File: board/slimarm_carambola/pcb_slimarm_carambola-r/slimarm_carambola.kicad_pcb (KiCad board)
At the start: 4 copper layers, 50 x 29.7 mm, 85 parts, among them J1 USB_C_Receptacle_USB2.0, J2 Conn_01x14_Pin, J3 Micro_SD_Card_Det2, J4 DF13A-7P-1.25H21, J5 Conn_01x03, U1 AT91SAM9G25-CU, U2 16bit-DDR2-8bank-FBGA84, U3 SY8089AAAC, U5 AMS1117, U7 XC6206PxxxMR, Y1 Crystal

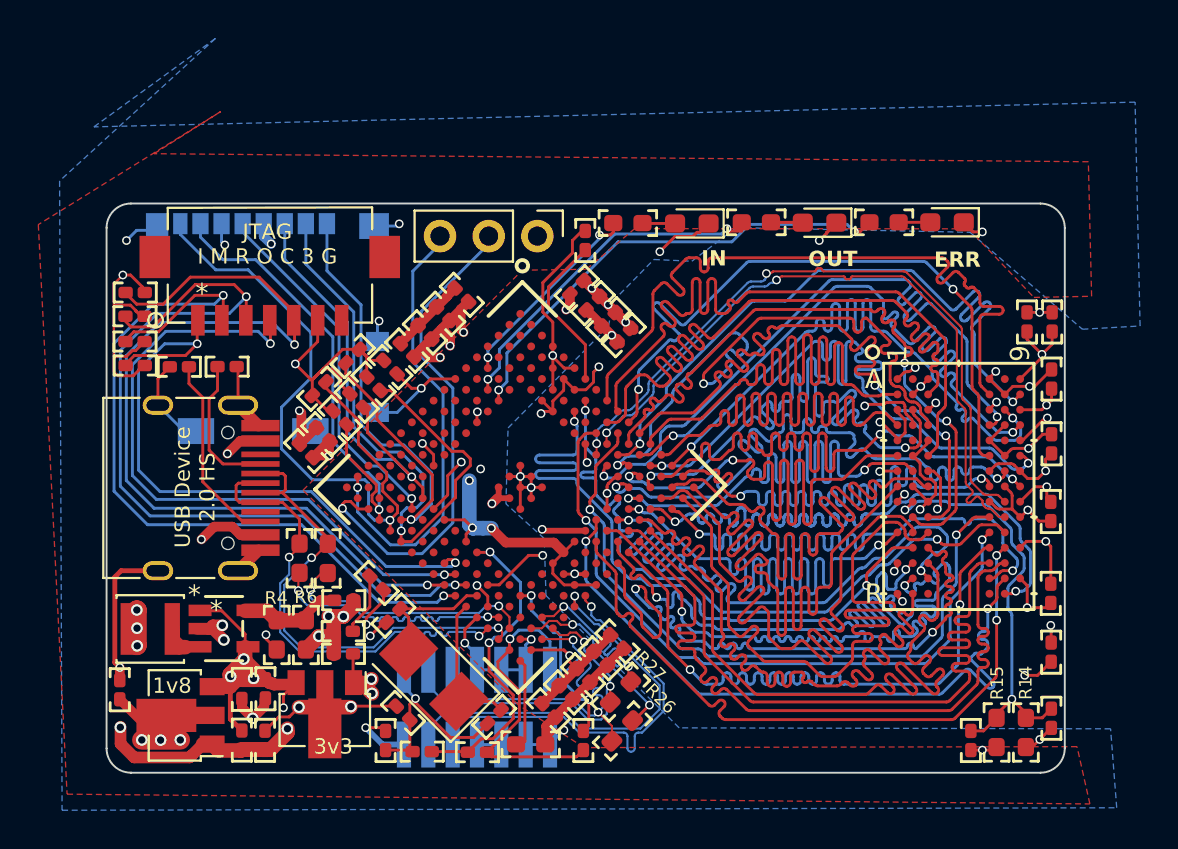
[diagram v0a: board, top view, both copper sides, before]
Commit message: 23x2c7-part2(Carambola)
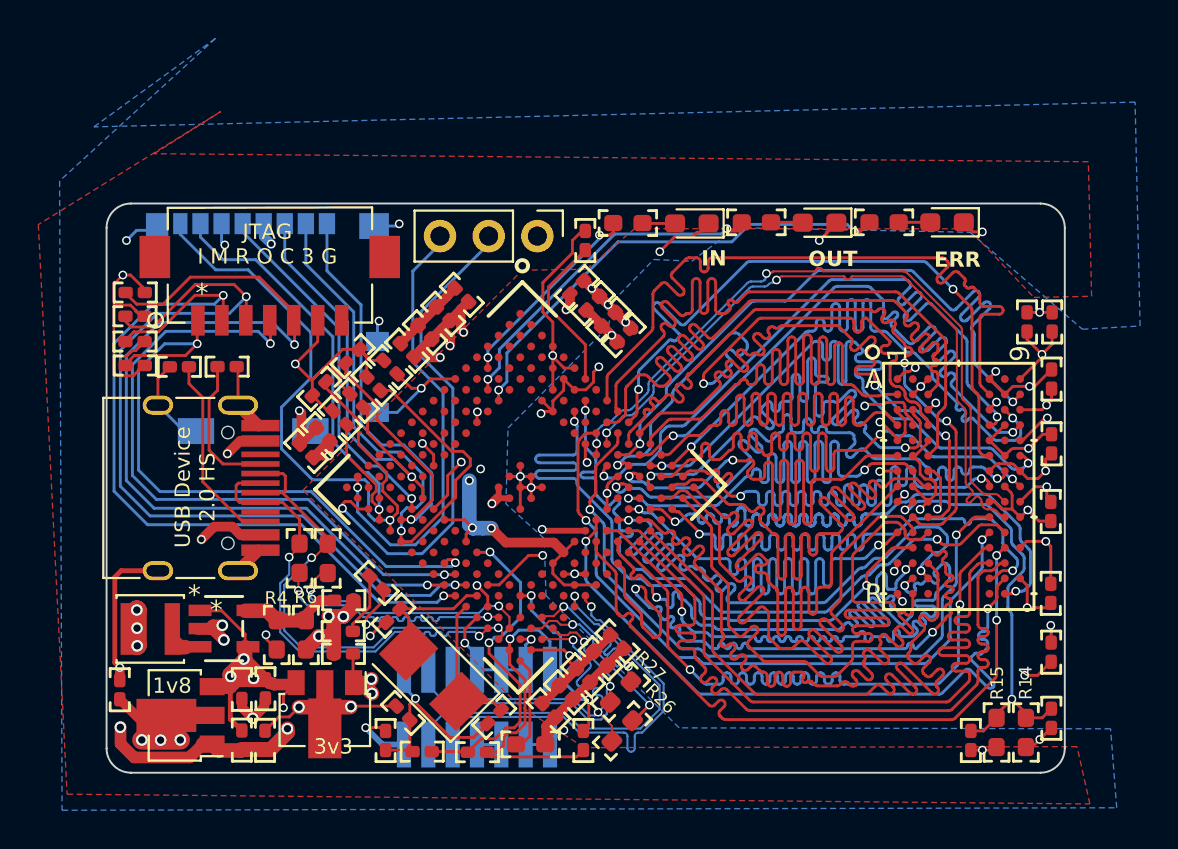
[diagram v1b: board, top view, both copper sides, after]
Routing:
- net /1v8_DDR: track 181.6 -> 180.1 mm
- net Net-(U1C-NRST): track 16.4 -> 17.0 mm
